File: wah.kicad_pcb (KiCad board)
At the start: 4 copper layers, 99.1 x 54.5 mm, 38 parts, among them J1 Barrel_Jack_Switch, J2 In, J3 Out, SW1 SW_Push_3PDT, U1 TL072, U2 L78L05_TO92

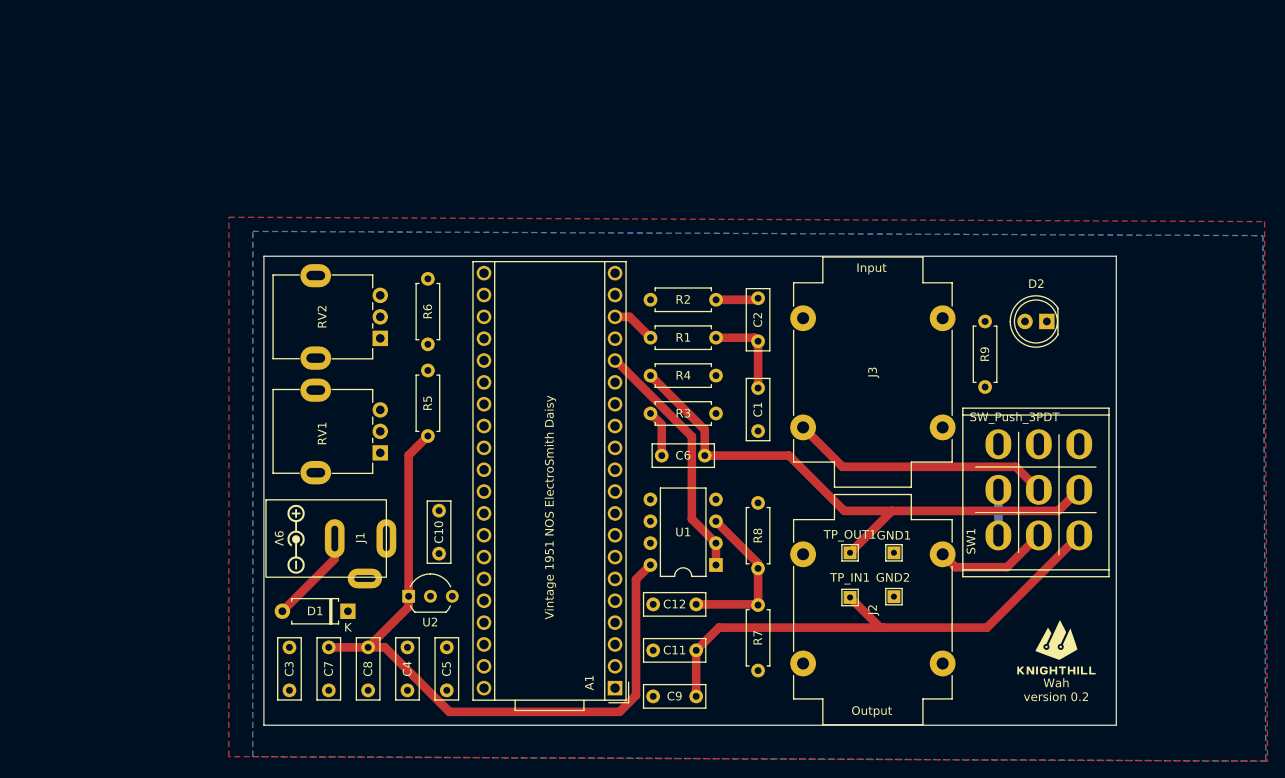
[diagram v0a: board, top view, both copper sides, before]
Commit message: fix errors
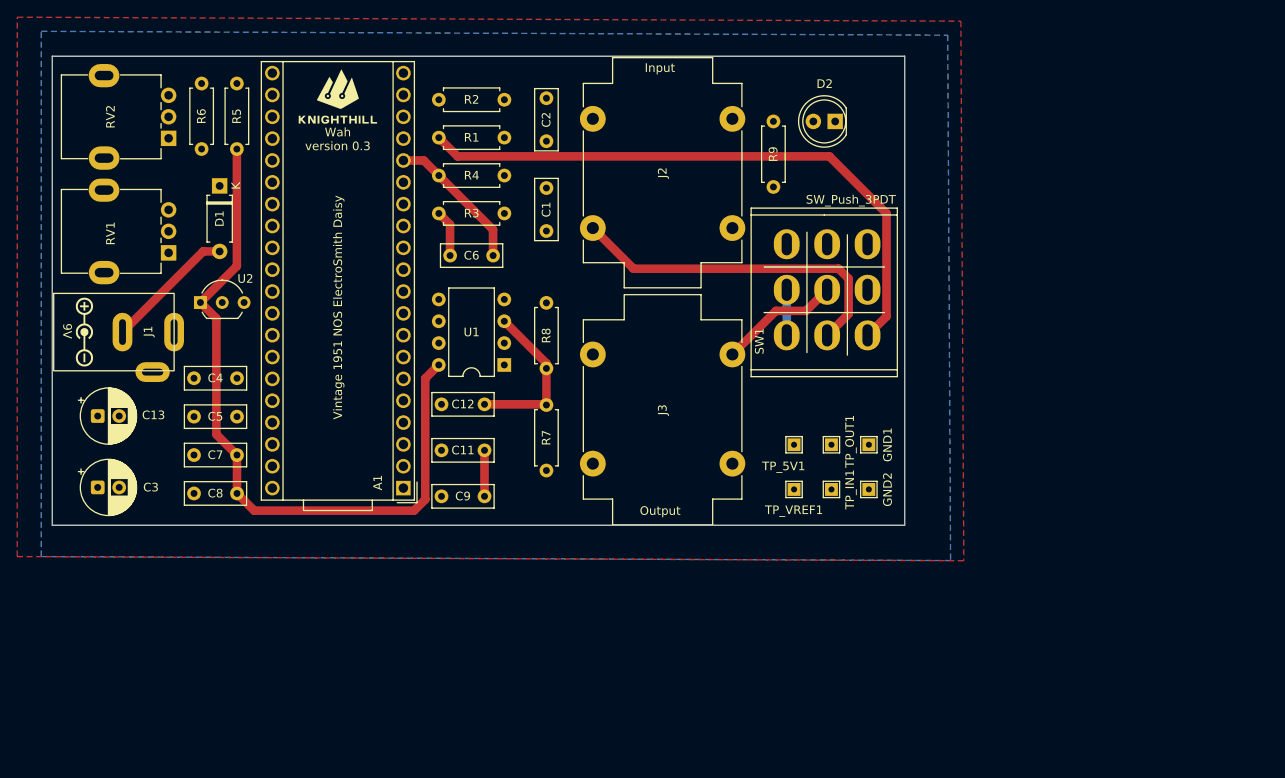
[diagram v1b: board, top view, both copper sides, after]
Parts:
- removed C10: 100u, Capacitor_THT:C_Rect_L7.0mm_W2.5mm_P5.00mm
- added C13: 100u, Capacitor_THT:CP_Radial_D6.3mm_P2.50mm, F.Cu at (47.7, 75.0)
- added TP_5V1: TestPoint, TestPoint:TestPoint_THTPad_1.5x1.5mm_Drill0.7mm, F.Cu at (128.7, 78.4)
- added TP_VREF1: TestPoint, TestPoint:TestPoint_THTPad_1.5x1.5mm_Drill0.7mm, F.Cu at (128.7, 83.6)
- C3: footprint Capacitor_THT:C_Rect_L7.0mm_W2.5mm_P5.00mm -> Capacitor_THT:CP_Radial_D6.3mm_P2.50mm
- moved G*** 105.3 mm to (75.5, 38.8)
- moved J2 55.6 mm to (105.3, 53.2), turned to 90 degrees
- moved D1 51.7 mm to (61.9, 48.3), turned to -90 degrees
- moved U2 41.9 mm to (59.6, 61.8)
- moved R5 40.1 mm to (63.9, 44.0)
- moved C4 37.1 mm to (63.9, 70.6), turned to 180 degrees
- moved C5 36.3 mm to (63.9, 75.1), turned to 180 degrees
- moved R6 34.8 mm to (59.8, 36.4)
- moved G*** 34.4 mm to (46.2, 65.3)
- moved J1 34.4 mm to (56.6, 65.3)
- moved SW1 33.9 mm to (132.2, 60.6)
- moved C6 33.9 mm to (88.7, 56.4)
- moved R4 33.9 mm to (87.4, 47.1)
- moved R8 33.9 mm to (99.9, 61.9)
- moved R9 33.9 mm to (126.3, 48.4)
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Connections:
- C11 pad 1: /FX_IN -> /AUDIO_OUT
- C6 pad 2: /FX_OUT -> /AUDIO_IN
- C9 pad 1: /FX_IN -> /AUDIO_OUT
- R1 pad 1: /AUDIO_OUT -> /FX_IN
- R4 pad 1: /FX_OUT -> /AUDIO_IN
- U1 pad 1: /AUDIO_IN -> /FX_OUT
- U1 pad 2: /AUDIO_IN -> /FX_OUT
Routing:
- net Net-(U1C-V+): track 83.0 -> 128.3 mm
- net /AUDIO_OUT: track 5.13 -> 48.0 mm
- net /FX_IN: track 60.7 -> 90.5 mm
- net Net-(J2-PadT): track 13.3 -> 39.8 mm
- net Net-(J3-PadT): track 30.4 -> 14.1 mm
- net /AUDIO_IN: track 28.7 -> 16.8 mm
- net Net-(D1-A): track 11.0 -> 15.2 mm
- net /FX_OUT: track 66.0 -> 63.7 mm
- net /POT1: track 16.5 -> 17.7 mm
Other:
- board text added: "Wah version 0.3"
- board text removed: "Wah version 0.2"
